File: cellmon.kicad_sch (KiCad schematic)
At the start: 13 parts, among them J1 Conn_01x02_Male, J2 Conn_01x02_Male, J3 Conn_01x06, J4 Conn_01x02_Male, U1 ATtiny85V-10S, U2 6N136

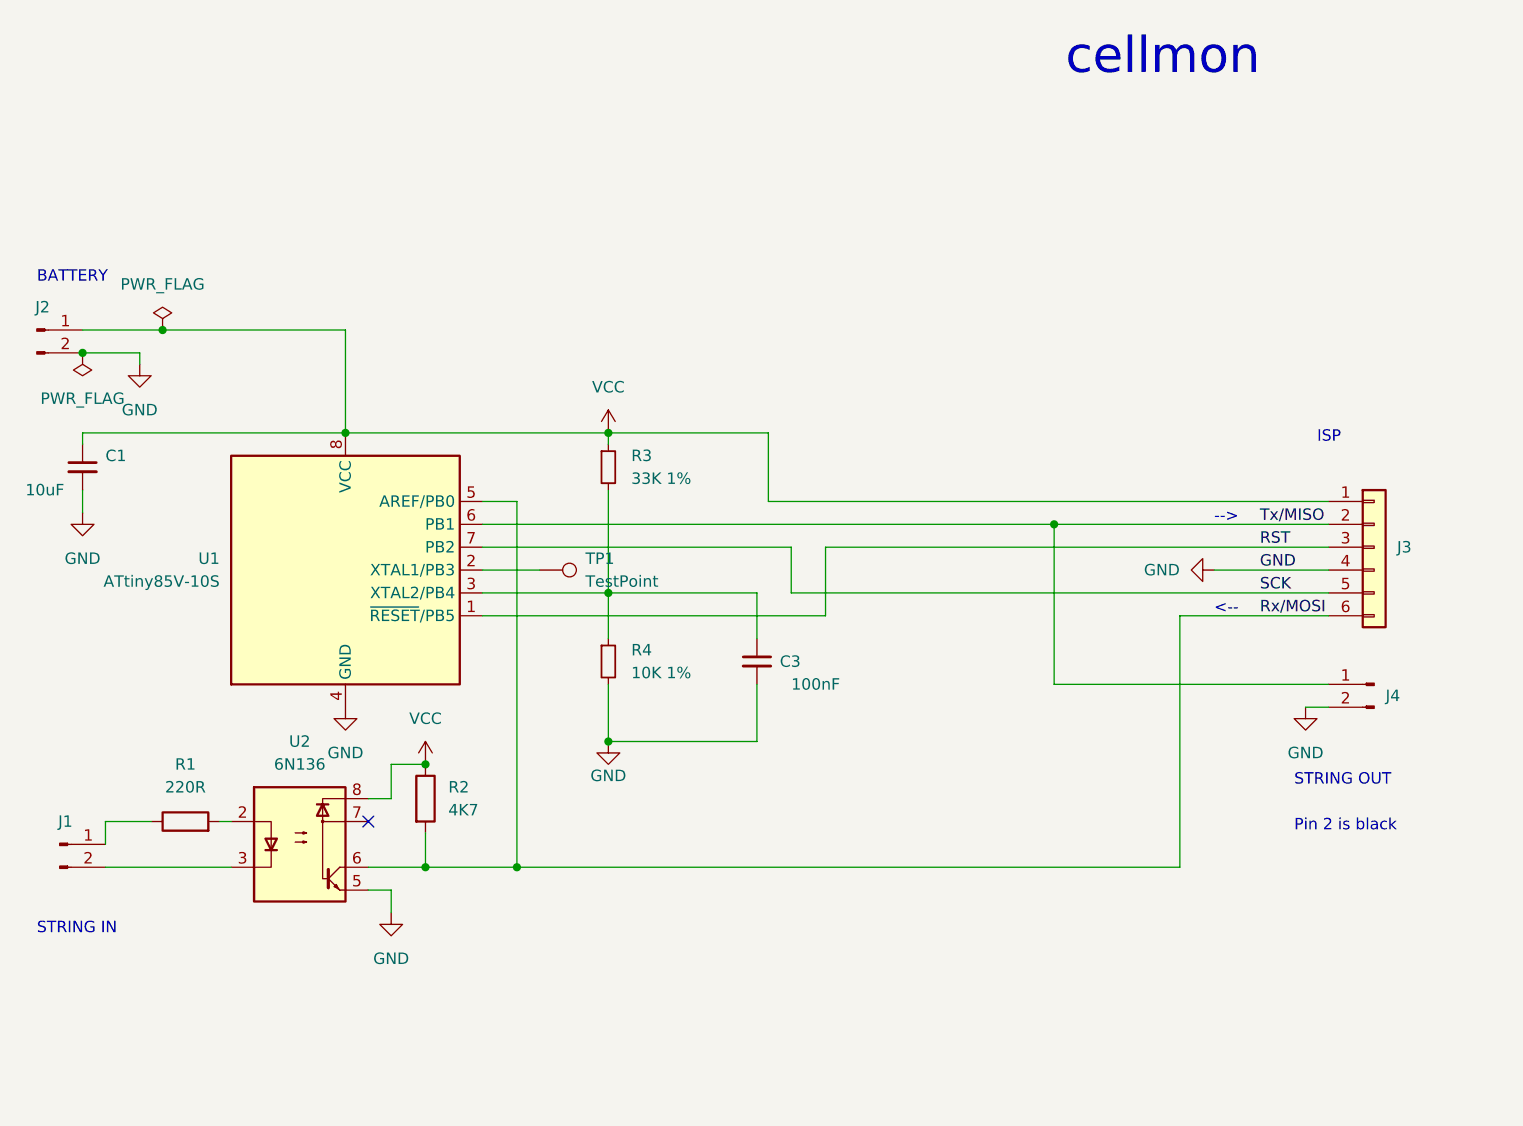
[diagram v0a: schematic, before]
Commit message: Update to R2 PCB
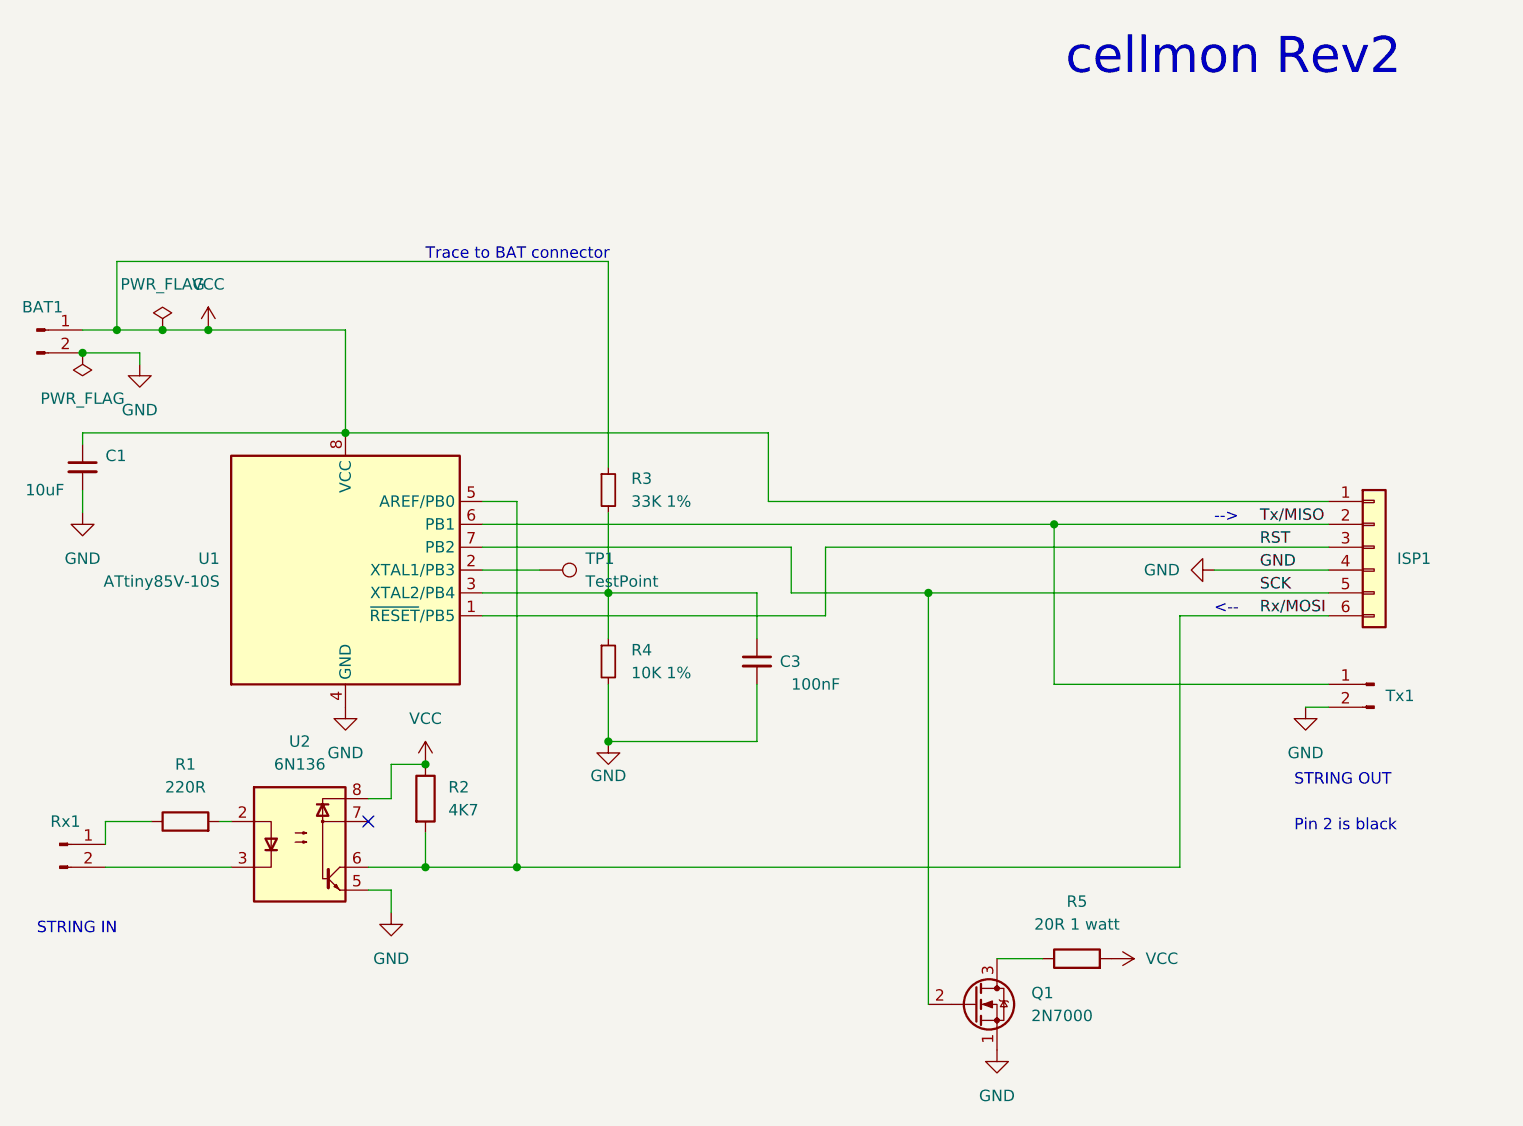
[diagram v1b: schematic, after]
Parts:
- added Q1: 2N7000, Package_TO_SOT_THT:TO-92_Inline, symbol Transistor_FET:2N7000
- added R5: 20R 1 watt, Resistor_THT:R_Axial_DIN0207_L6.3mm_D2.5mm_P10.16mm_Horizontal, symbol Device:R
- renumbered J2 to BAT1, J3 to ISP1, J1 to Rx1, J4 to Tx1
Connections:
- net GND: now also Q1.1 (S)
- net SCK: now also Q1.2 (G)
- net VCC: now also R5.2
- new net: Q1.3 (D), R5.1
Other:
- note added: "Trace to BAT connector"
- note added: "cellmon Rev2"
- note removed: "BATTERY"
- note removed: "ISP"
- note removed: "cellmon"
- moved on the sheet: R3

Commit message: R2 PCB
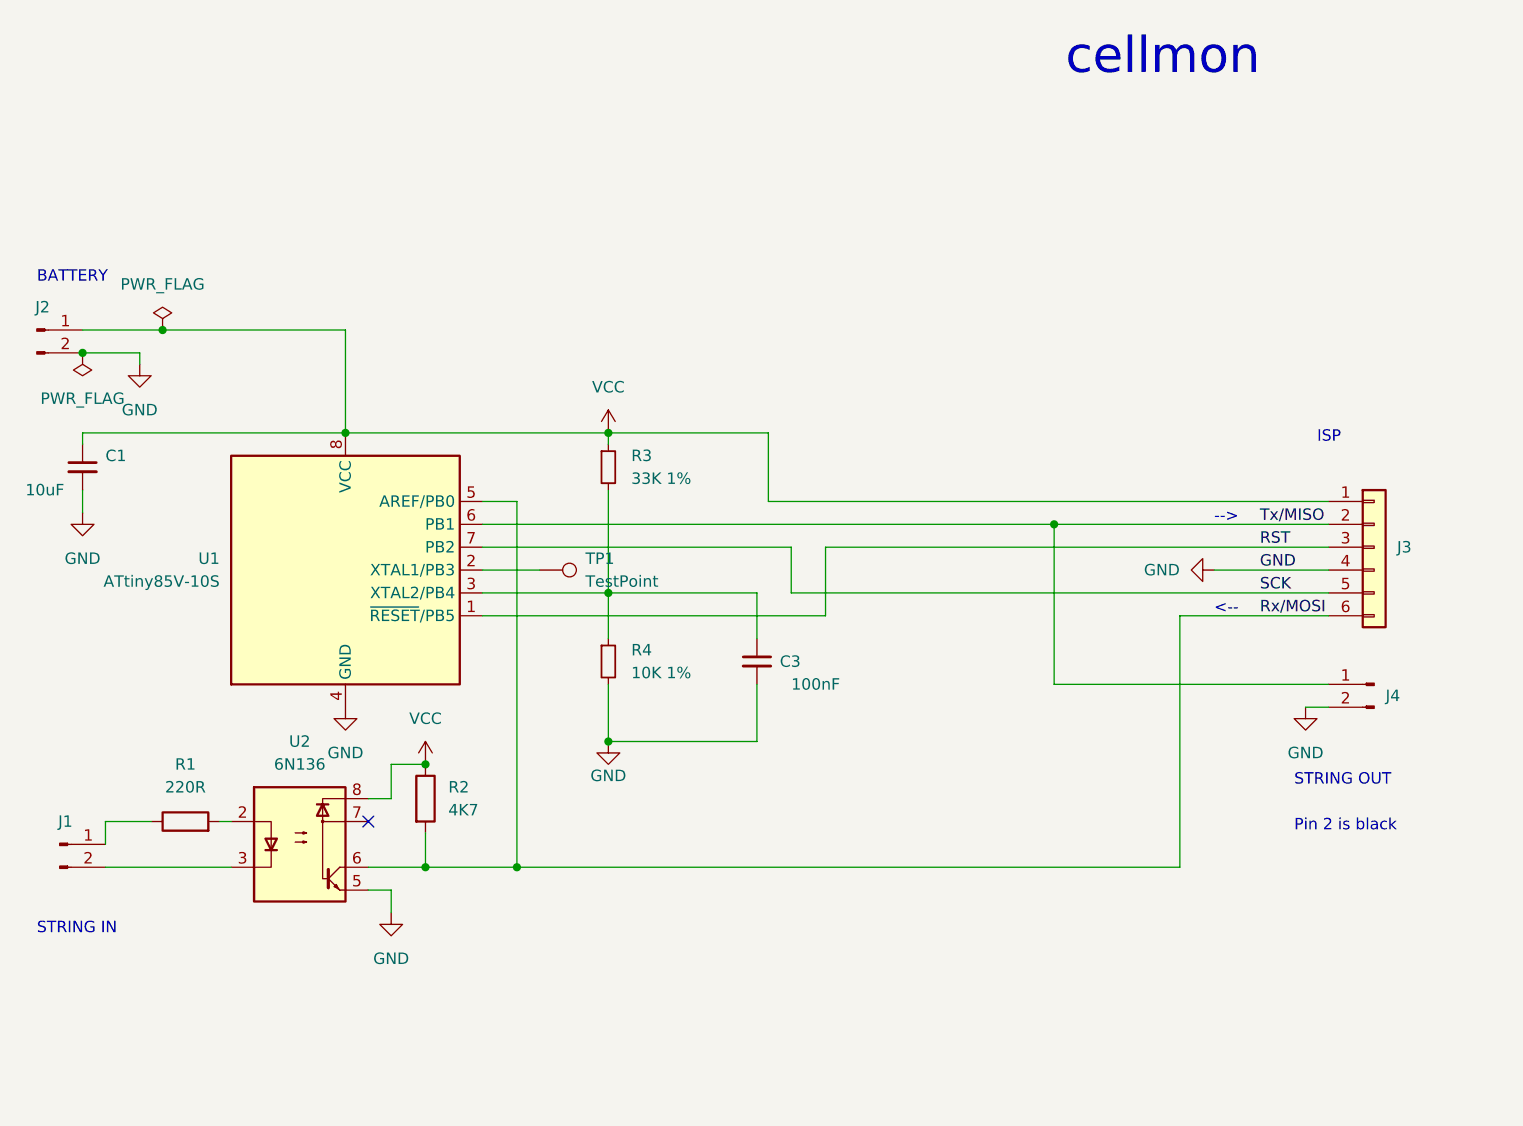
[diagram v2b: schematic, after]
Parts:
- removed Q1: 2N7000, Package_TO_SOT_THT:TO-92_Inline, symbol Transistor_FET:2N7000
- removed R5: 20R 1 watt, Resistor_THT:R_Axial_DIN0207_L6.3mm_D2.5mm_P10.16mm_Horizontal, symbol Device:R
- renumbered Rx1 to J1, BAT1 to J2, ISP1 to J3, Tx1 to J4
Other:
- note added: "BATTERY"
- note added: "ISP"
- note added: "cellmon"
- note removed: "Trace to BAT connector"
- note removed: "cellmon Rev2"
- moved on the sheet: R3
